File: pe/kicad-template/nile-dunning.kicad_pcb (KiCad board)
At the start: 2 copper layers, 7 parts, among them U2 TPS562202

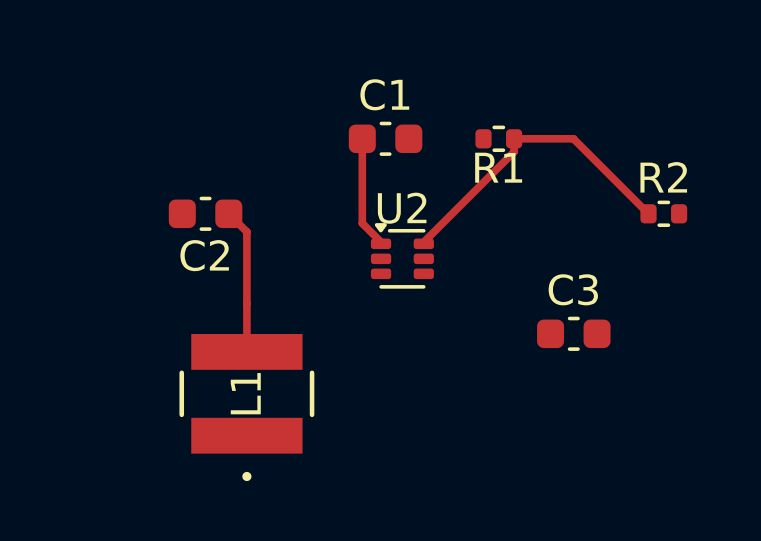
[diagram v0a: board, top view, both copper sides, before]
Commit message: incomplete but submit
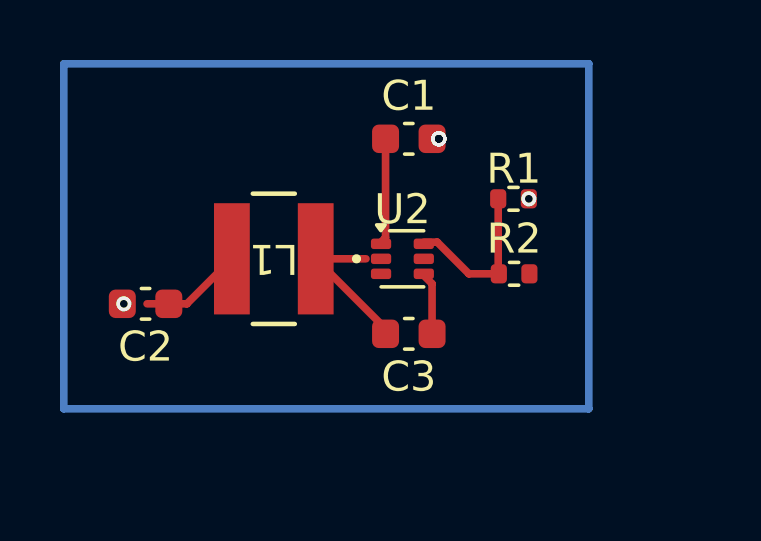
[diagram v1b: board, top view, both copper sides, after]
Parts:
- moved C3 5.50 mm to (155.5, 98.5), turned to 180 degrees
- moved R2 5.38 mm to (159.0, 96.5)
- moved L1 4.59 mm to (151.0, 96.0), turned to 180 degrees
- moved C2 3.61 mm to (146.7, 97.5)
- moved R1 2.06 mm to (159.0, 94.0), turned to 0 degrees
- moved C1 0.78 mm to (155.5, 92.0)
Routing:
- net Net-(U2-SW): track 0.00 -> 5.31 mm
- net Net-(U2-VFB): track 10.2 -> 5.45 mm
- net Net-(U2-VBST): track 0.00 -> 2.06 mm
- net +5V: track 4.85 -> 3.05 mm
- net GND: track 0.00 -> 0.28 mm, vias 0 -> 5
- added copper zone on B.Cu, net GND
